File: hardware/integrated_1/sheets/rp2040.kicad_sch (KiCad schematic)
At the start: 31 parts, among them SW2 DNF, SW3 DNF, U3 W25Q16JV, U4 RP2040, U5 FT24C04A, Y1 12MHz

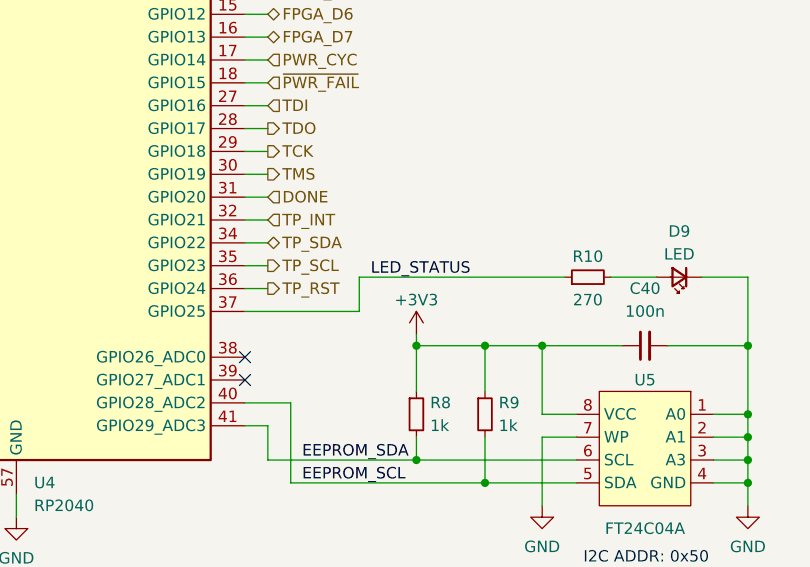
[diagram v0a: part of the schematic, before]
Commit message: exported 3d models + added date stamp
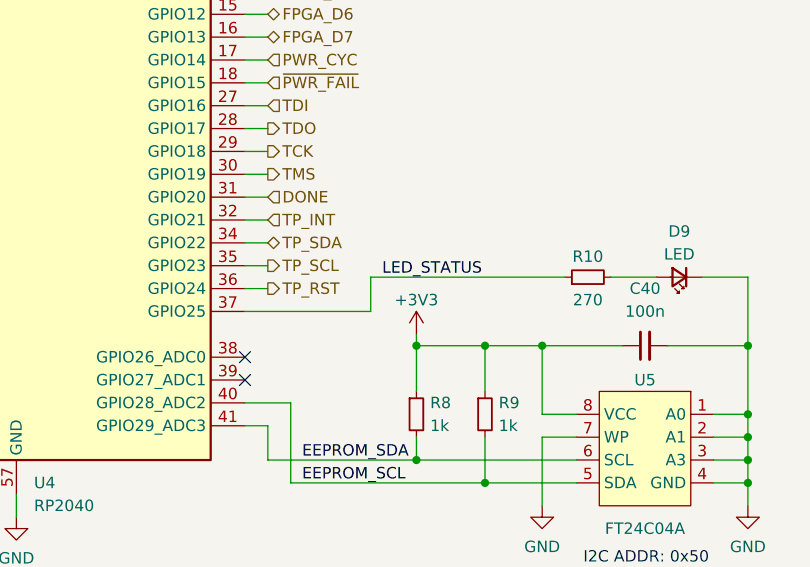
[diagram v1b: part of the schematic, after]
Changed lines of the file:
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@@
 	(wire
 		(pts
-			(xy 173.99 134.62) (xy 186.69 134.62)
+			(xy 173.99 134.62) (xy 187.96 134.62)
 		)
 		(stroke
@@
 	(wire
 		(pts
-			(xy 186.69 130.81) (xy 186.69 134.62)
+			(xy 187.96 130.81) (xy 187.96 134.62)
 		)
 		(stroke
@@
 	(wire
 		(pts
-			(xy 186.69 130.81) (xy 209.55 130.81)
+			(xy 187.96 130.81) (xy 209.55 130.81)
 		)
 		(stroke
@@
 	)
 	(label "LED_STATUS"
-		(at 187.96 130.81 0)
+		(at 189.23 130.81 0)
 		(fields_autoplaced yes)
 		(effects
